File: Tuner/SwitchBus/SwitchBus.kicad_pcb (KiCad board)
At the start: 2 copper layers, 100 x 100 mm, 80 parts, among them J1 Conn_01x01, J10 Conn_Coaxial, J11 Conn_Coaxial, J12 Conn_Coaxial, J13 Conn_01x01, J14 Conn_01x01, J15 Conn_01x01, J16 Conn_Coaxial, J17 Conn_02x10_Odd_Even, J2 Conn_Coaxial, J3 Conn_Coaxial, J4 Conn_Coaxial, J5 Conn_Coaxial, J6 Conn_Coaxial, J7 Conn_Coaxial, J8 Conn_Coaxial, J9 Conn_Coaxial

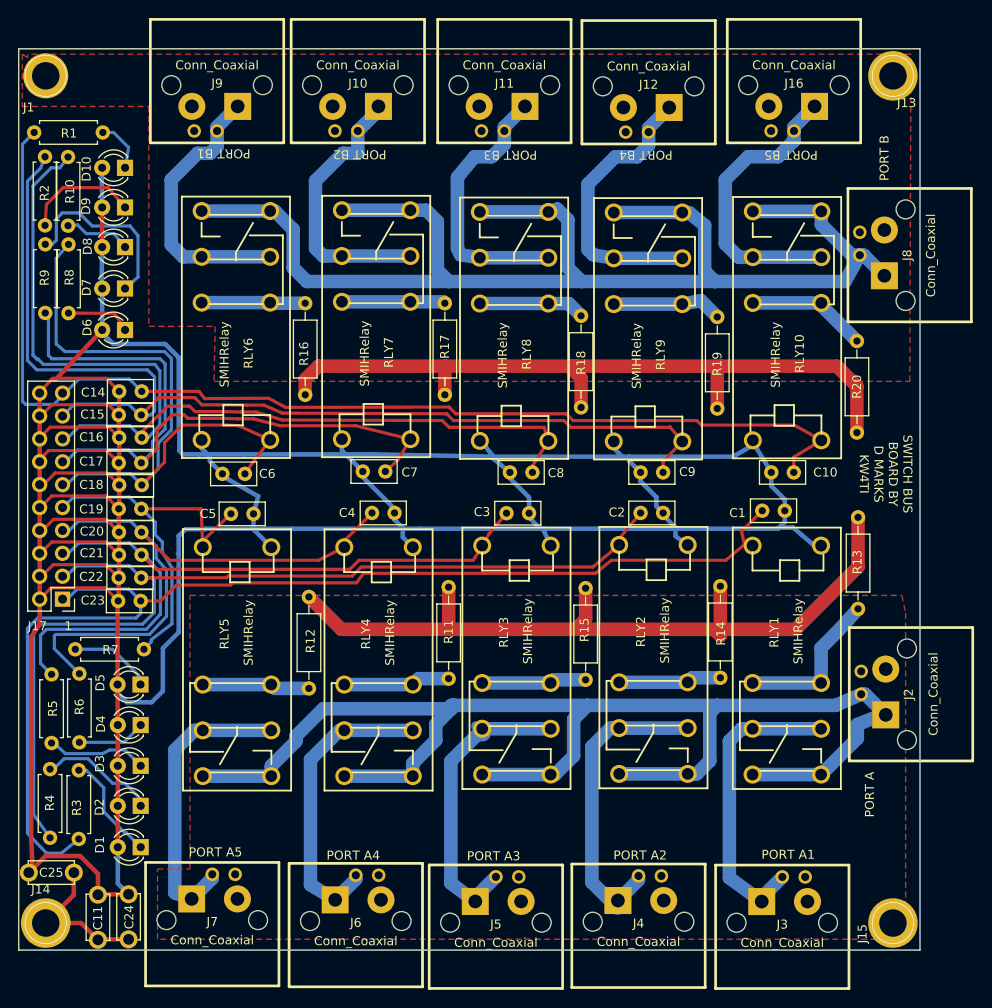
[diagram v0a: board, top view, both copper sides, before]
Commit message: Documentation update
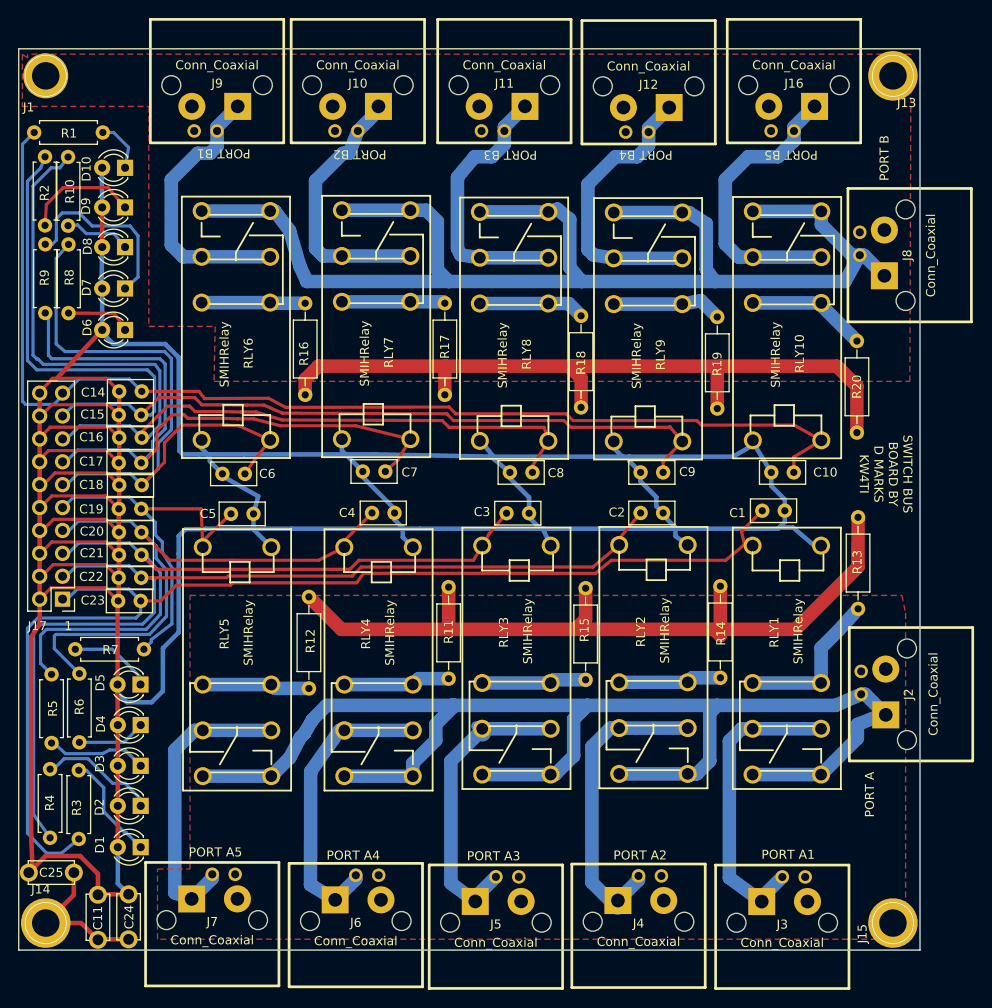
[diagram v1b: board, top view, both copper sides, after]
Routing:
- net Net-(J10-Pad1): track 30.5 -> 29.7 mm
- net Net-(J8-Pad1): track 152.8 -> 152.3 mm
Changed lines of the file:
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@@
   (segment (start 53 147) (end 56.9316 147) (width 0.5) (layer F.Cu) (net 22) (status 10))
   (segment (start 56.9316 147) (end 58.79084 148.85924) (width 0.5) (layer F.Cu) (net 22) (status 20))
-  (segment (start 78.025 130.7) (end 78.025 129.575) (width 1.5) (layer B.Cu) (net 23))
-  (segment (start 98.005 123.22) (end 98.005 122.85) (width 1.5) (layer B.Cu) (net 23))
-  (segment (start 83.81 123.22) (end 98.005 123.22) (width 1.5) (layer B.Cu) (net 23))
-  (segment (start 80.75 126.28) (end 83.81 123.22) (width 1.5) (layer B.Cu) (net 23))
-  (segment (start 80.75 126.85) (end 80.75 126.28) (width 1.5) (layer B.Cu) (net 23))
-  (segment (start 78.025 129.575) (end 80.75 126.85) (width 1.5) (layer B.Cu) (net 23))
+  (segment (start 98.375 122.85) (end 84.1473 122.85) (width 1.5) (layer B.Cu) (net 23))
+  (segment (start 80.0862 128.6388) (end 78.025 130.7) (width 1.5) (layer B.Cu) (net 23))
+  (segment (start 81.2546 126.4031) (end 80.0862 128.6388) (width 1.5) (layer B.Cu) (net 23))
+  (segment (start 81.7118 125.9459) (end 81.2546 126.4031) (width 1.5) (layer B.Cu) (net 23))
+  (segment (start 82.6008 124.4346) (end 81.7118 125.9459) (width 1.5) (layer B.Cu) (net 23))
+  (segment (start 84.1473 122.85) (end 82.6008 124.4346) (width 1.5) (layer B.Cu) (net 23))
   (segment (start 93.725 130.7) (end 93.725 129.275) (width 1.5) (layer B.Cu) (net 23))
   (segment (start 93.725 129.275) (end 96.275 126.725) (width 1.5) (layer B.Cu) (net 23))
@@
   (segment (start 87.4014 142.1384) (end 85.1154 144.4244) (width 1.5) (layer B.Cu) (net 28) (status 30))
   (segment (start 86.125 125.62) (end 85.605 125.62) (width 1.5) (layer B.Cu) (net 28))
-  (segment (start 85.605 125.62) (end 82.375 128.85) (width 1.5) (layer B.Cu) (net 28))
+  (segment (start 85.605 125.62) (end 82.3976 130.1877) (width 1.5) (layer B.Cu) (net 28))
   (segment (start 82.375 142.759) (end 85.1154 144.4244) (width 1.5) (layer B.Cu) (net 28) (status 20))
-  (segment (start 82.375 128.85) (end 82.375 142.759) (width 1.5) (layer B.Cu) (net 28))
+  (segment (start 82.3976 130.1877) (end 82.375 142.759) (width 1.5) (layer B.Cu) (net 28))
   (segment (start 86.125 125.62) (end 86.125 125.7) (width 2) (layer B.Cu) (net 28) (status 30))
   (segment (start 86.314 125.273) (end 86.68216 125.273) (width 1) (layer B.Cu) (net 28) (status 30))
@@
   (segment (start 142.4305 72.898) (end 139.055 69.5225) (width 1.5) (layer B.Cu) (net 30))
   (segment (start 77.9 68) (end 78.414 68) (width 1.5) (layer B.Cu) (net 30))
-  (segment (start 78.414 68) (end 80.4545 70.0405) (width 1.5) (layer B.Cu) (net 30))
+  (segment (start 78.414 68) (end 80.0481 70.1548) (width 1.5) (layer B.Cu) (net 30))
   (segment (start 81.9785 75.819) (end 97.7265 75.819) (width 1.5) (layer B.Cu) (net 30))
-  (segment (start 80.4545 74.295) (end 81.9785 75.819) (width 1.5) (layer B.Cu) (net 30))
-  (segment (start 80.4545 70.0405) (end 80.4545 74.295) (width 1.5) (layer B.Cu) (net 30))
+  (segment (start 81.2165 74.1553) (end 81.9785 75.819) (width 1.5) (layer B.Cu) (net 30))
+  (segment (start 80.0481 70.1548) (end 81.2165 74.1553) (width 1.5) (layer B.Cu) (net 30))
   (segment (start 93.462 67.912) (end 95.217 67.912) (width 1.5) (layer B.Cu) (net 30))
   (segment (start 97.7265 75.819) (end 112.4585 75.819) (width 1.5) (layer B.Cu) (net 30))
@@
   (segment (start 95.217 67.912) (end 96.4565 69.1515) (width 1.5) (layer B.Cu) (net 30))
   (segment (start 108.7655 68.1025) (end 109.7585 67.785) (width 1.5) (layer B.Cu) (net 30) (status 10))
-  (segment (start 109.7585 67.785) (end 110.9345 68.961) (width 1.5) (layer B.Cu) (net 30))
-  (segment (start 110.9345 68.961) (end 110.9345 74.295) (width 1.5) (layer B.Cu) (net 30))
-  (segment (start 110.9345 74.295) (end 112.4585 75.819) (width 1.5) (layer B.Cu) (net 30))
+  (segment (start 109.7585 67.785) (end 111.1377 68.9229) (width 1.5) (layer B.Cu) (net 30))
+  (segment (start 111.1377 68.9229) (end 111.1377 74.2569) (width 1.5) (layer B.Cu) (net 30))
+  (segment (start 111.1377 74.2569) (end 112.4585 75.819) (width 1.5) (layer B.Cu) (net 30))
   (segment (start 112.4585 75.819) (end 127.254 75.819) (width 1.5) (layer B.Cu) (net 30))
   (segment (start 123.6245 68.166) (end 124.3635 68.166) (width 1.5) (layer B.Cu) (net 30) (status 30))
-  (segment (start 124.3635 68.166) (end 126.111 69.596) (width 1.5) (layer B.Cu) (net 30) (status 10))
-  (segment (start 126.111 69.596) (end 126.111 74.676) (width 1.5) (layer B.Cu) (net 30))
-  (segment (start 126.111 74.676) (end 127.254 75.819) (width 1.5) (layer B.Cu) (net 30))
+  (segment (start 124.3635 68.166) (end 126.2888 69.4055) (width 1.5) (layer B.Cu) (net 30) (status 10))
+  (segment (start 126.2888 69.4055) (end 126.2888 74.4855) (width 1.5) (layer B.Cu) (net 30))
+  (segment (start 126.2888 74.4855) (end 127.254 75.819) (width 1.5) (layer B.Cu) (net 30))
   (segment (start 141.671 75.819) (end 143.322 72.898) (width 1.5) (layer B.Cu) (net 30) (status 20))
   (segment (start 127.254 75.819) (end 141.671 75.819) (width 1.5) (layer B.Cu) (net 30))
@@
   (segment (start 89.916 56.83) (end 87.63 59.116) (width 1.5) (layer B.Cu) (net 37))
   (segment (start 85.862 72.992) (end 83.787 72.992) (width 1.5) (layer B.Cu) (net 37))
-  (segment (start 87.63 61.595) (end 87.63 59.116) (width 1.5) (layer B.Cu) (net 37))
-  (segment (start 85.979 61.595) (end 87.63 61.595) (width 1.5) (layer B.Cu) (net 37))
+  (segment (start 86.6648 61.58992) (end 87.63 59.116) (width 1.5) (layer B.Cu) (net 37) (status 800000))
+  (segment (start 85.979 61.595) (end 86.6648 61.58992) (width 1.5) (layer B.Cu) (net 37))
   (segment (start 82.931 64.643) (end 85.979 61.595) (width 1.5) (layer B.Cu) (net 37))
   (segment (start 82.931 72.136) (end 82.931 64.643) (width 1.5) (layer B.Cu) (net 37))

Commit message: Added some fixes to tuner code
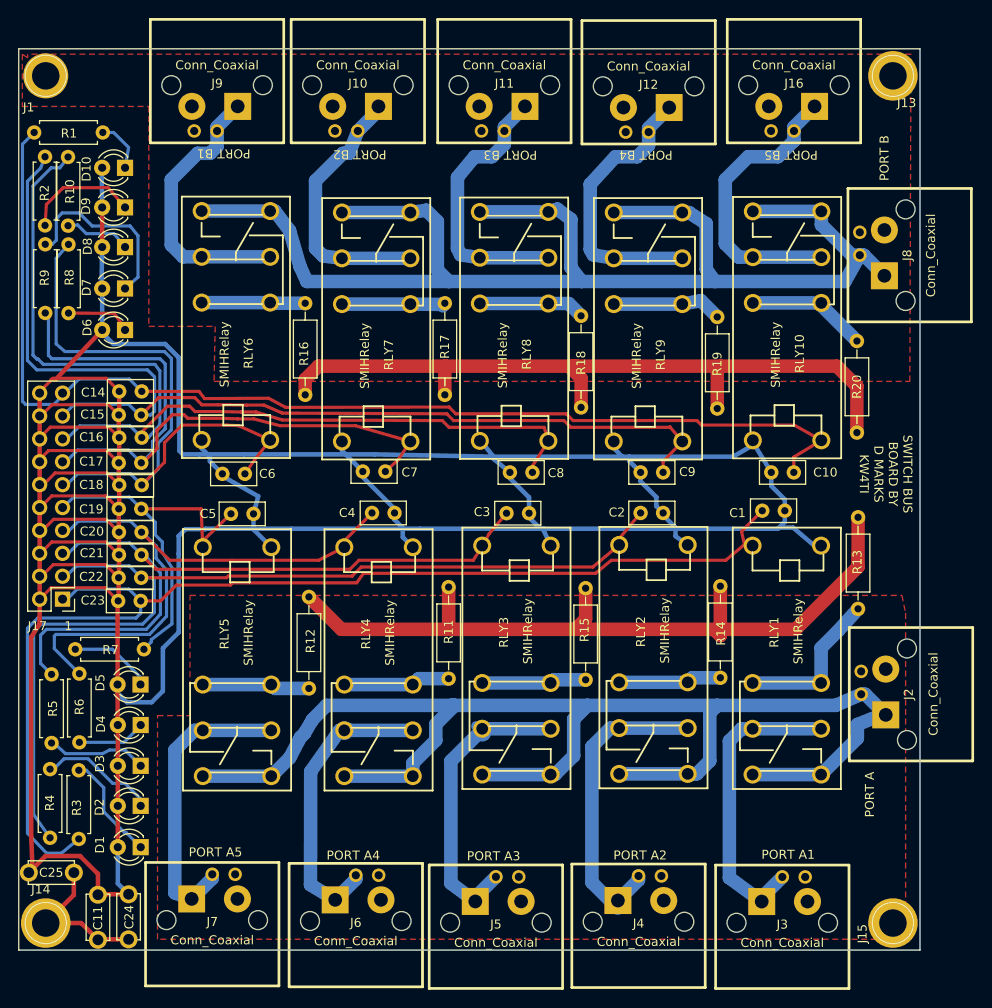
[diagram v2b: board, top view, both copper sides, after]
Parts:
- moved RLY7 0.25 mm to (89.7, 83.6)
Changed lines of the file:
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@@
   )
   (setup
-    (last_trace_width 1.5)
+    (last_trace_width 0.25)
     (user_trace_width 0.35)
     (user_trace_width 0.5)
@@
   )
   (module tuner:SMIHRelay (layer F.Cu)
-    (at 89.662 83.312 90)
+    (at 89.662 83.566 90)
     (fp_text reference RLY7 (at -0.381 1.397 90) (layer F.SilkS)
       (effects (font (size 1 1) (thickness 0.15)))
@@
   (segment (start 76.073 91.059) (end 78.994 91.821) (width 0.35) (layer F.Cu) (net 7))
   (segment (start 90.678 96.901) (end 92.075 95.631) (width 0.35) (layer F.Cu) (net 7) (status 10))
-  (segment (start 92.075 95.631) (end 93.462 93.312) (width 0.35) (layer F.Cu) (net 7) (status 20))
-  (segment (start 87.376 91.821) (end 93.462 93.312) (width 0.35) (layer F.Cu) (net 7) (status 20))
+  (segment (start 92.075 95.631) (end 93.462 93.566) (width 0.35) (layer F.Cu) (net 7) (status 20))
+  (segment (start 87.376 91.821) (end 93.462 93.566) (width 0.35) (layer F.Cu) (net 7) (status 20))
   (segment (start 72.62 91) (end 74.295 91.059) (width 0.35) (layer F.Cu) (net 7))
   (segment (start 52.9463 79.3115) (end 52.9463 79.2861) (width 0.35) (layer F.Cu) (net 7) (status 30))
@@
   (segment (start 104.5 97.642) (end 104.5 97) (width 0.5) (layer B.Cu) (net 9))
   (segment (start 106.625 101.525) (end 106.625 101.625) (width 0.5) (layer B.Cu) (net 9))
-  (segment (start 85.862 93.312) (end 85.862 94.585) (width 0.5) (layer B.Cu) (net 9))
+  (segment (start 85.862 93.566) (end 85.862 94.585) (width 0.5) (layer B.Cu) (net 9) (status 10))
   (segment (start 85.862 94.585) (end 88.178 96.901) (width 0.5) (layer B.Cu) (net 9))
   (segment (start 71.21 95.25) (end 71.21 95.77) (width 0.5) (layer B.Cu) (net 9))
@@
   (segment (start 81.2165 74.1553) (end 81.9785 75.819) (width 1.5) (layer B.Cu) (net 30))
   (segment (start 80.0481 70.1548) (end 81.2165 74.1553) (width 1.5) (layer B.Cu) (net 30))
-  (segment (start 93.462 67.912) (end 95.217 67.912) (width 1.5) (layer B.Cu) (net 30))
+  (segment (start 93.462 68.166) (end 95.217 67.912) (width 1.5) (layer B.Cu) (net 30) (status 10))
   (segment (start 97.7265 75.819) (end 112.4585 75.819) (width 1.5) (layer B.Cu) (net 30))
   (segment (start 96.4565 74.549) (end 97.7265 75.819) (width 1.5) (layer B.Cu) (net 30))
@@
   (segment (start 95.217 67.912) (end 96.4565 69.1515) (width 1.5) (layer B.Cu) (net 30))
   (segment (start 108.7655 68.1025) (end 109.7585 67.785) (width 1.5) (layer B.Cu) (net 30) (status 10))
-  (segment (start 109.7585 67.785) (end 111.1377 68.9229) (width 1.5) (layer B.Cu) (net 30))
-  (segment (start 111.1377 68.9229) (end 111.1377 74.2569) (width 1.5) (layer B.Cu) (net 30))
-  (segment (start 111.1377 74.2569) (end 112.4585 75.819) (width 1.5) (layer B.Cu) (net 30))
+  (segment (start 109.7585 67.785) (end 111.2647 68.9229) (width 1.5) (layer B.Cu) (net 30))
+  (segment (start 111.2647 68.9229) (end 111.2647 74.2569) (width 1.5) (layer B.Cu) (net 30))
+  (segment (start 111.2647 74.2569) (end 112.4585 75.819) (width 1.5) (layer B.Cu) (net 30))
   (segment (start 112.4585 75.819) (end 127.254 75.819) (width 1.5) (layer B.Cu) (net 30))
   (segment (start 123.6245 68.166) (end 124.3635 68.166) (width 1.5) (layer B.Cu) (net 30) (status 30))
@@
   (segment (start 116.0245 68.166) (end 123.6245 68.166) (width 1.5) (layer B.Cu) (net 30) (status 30))
   (segment (start 101.1655 68.1025) (end 108.7655 68.1025) (width 1.5) (layer B.Cu) (net 30) (status 30))
-  (segment (start 85.862 67.912) (end 93.462 67.912) (width 1.5) (layer B.Cu) (net 30))
+  (segment (start 85.862 68.166) (end 93.462 68.166) (width 1.5) (layer B.Cu) (net 30) (status 30))
   (segment (start 70.3 68) (end 77.9 68) (width 1.5) (layer B.Cu) (net 30))
   (segment (start 97.7 119.885) (end 94.38 119.885) (width 1.5) (layer B.Cu) (net 31))
@@
   (segment (start 66.929 71.755) (end 66.929 64.516) (width 1.5) (layer B.Cu) (net 36))
   (segment (start 68.254 73.08) (end 66.929 71.755) (width 1.5) (layer B.Cu) (net 36))
-  (segment (start 93.462 72.992) (end 85.862 72.992) (width 1.5) (layer B.Cu) (net 37))
+  (segment (start 93.462 73.246) (end 85.862 73.246) (width 1.5) (layer B.Cu) (net 37) (status 30))
   (segment (start 89.916 56.388) (end 89.916 56.83) (width 1.5) (layer B.Cu) (net 37))
   (segment (start 89.916 56.83) (end 87.63 59.116) (width 1.5) (layer B.Cu) (net 37))
-  (segment (start 85.862 72.992) (end 83.787 72.992) (width 1.5) (layer B.Cu) (net 37))
-  (segment (start 86.6648 61.58992) (end 87.63 59.116) (width 1.5) (layer B.Cu) (net 37) (status 800000))
+  (segment (start 85.862 73.246) (end 83.787 72.992) (width 1.5) (layer B.Cu) (net 37) (status 10))
+  (segment (start 86.6648 61.58992) (end 87.63 59.116) (width 1.5) (layer B.Cu) (net 37))
   (segment (start 85.979 61.595) (end 86.6648 61.58992) (width 1.5) (layer B.Cu) (net 37))
   (segment (start 82.931 64.643) (end 85.979 61.595) (width 1.5) (layer B.Cu) (net 37))
@@
   (segment (start 118.618 61.976) (end 119.888 60.706) (width 1.5) (layer B.Cu) (net 39))
   (segment (start 116.205 61.976) (end 118.618 61.976) (width 1.5) (layer B.Cu) (net 39))
-  (segment (start 113.157 65.024) (end 116.205 61.976) (width 1.5) (layer B.Cu) (net 39))
-  (segment (start 113.157 72.263) (end 113.157 65.024) (width 1.5) (layer B.Cu) (net 39))
-  (segment (start 113.759 72.865) (end 113.157 72.263) (width 1.5) (layer B.Cu) (net 39))
+  (segment (start 113.411 65.024) (end 116.205 61.976) (width 1.5) (layer B.Cu) (net 39))
+  (segment (start 113.411 72.263) (end 113.411 65.024) (width 1.5) (layer B.Cu) (net 39))
+  (segment (start 113.759 72.865) (end 113.411 72.263) (width 1.5) (layer B.Cu) (net 39))
   (segment (start 139.055 73.119) (end 131.455 73.119) (width 1.5) (layer B.Cu) (net 40))
   (segment (start 136.017 59.116) (end 136.017 58.674) (width 1.5) (layer B.Cu) (net 40))
@@
   (segment (start 77.972 78.232) (end 77.9 78.16) (width 1.5) (layer B.Cu) (net 41))
   (segment (start 70.3 78.16) (end 77.9 78.16) (width 1.5) (layer B.Cu) (net 41))
-  (segment (start 93.462 78.072) (end 97.122 78.072) (width 1.5) (layer B.Cu) (net 42))
-  (segment (start 97.122 78.072) (end 97.282 78.232) (width 1.5) (layer B.Cu) (net 42))
-  (segment (start 85.862 78.072) (end 93.462 78.072) (width 1.5) (layer B.Cu) (net 42))
+  (segment (start 93.462 78.326) (end 96.901 78.359) (width 1.5) (layer B.Cu) (net 42) (status 10))
+  (segment (start 96.901 78.359) (end 97.061 78.519) (width 1.5) (layer B.Cu) (net 42))
+  (segment (start 85.862 78.326) (end 93.462 78.326) (width 1.5) (layer B.Cu) (net 42) (status 30))
   (segment (start 108.7655 78.2625) (end 111.0285 78.2625) (width 1.5) (layer B.Cu) (net 43))
   (segment (start 111.0285 78.2625) (end 112.395 79.629) (width 1.5) (layer B.Cu) (net 43))
@@
     (polygon
       (pts
-        (xy 148.4 112.6) (xy 148.4 148.8) (xy 65.4 148.8) (xy 65.4 141) (xy 69 141)
+        (xy 148.4 112.6) (xy 148.4 148.8) (xy 65.4 148.8) (xy 65.4 123.982) (xy 69 123.982)
         (xy 69 110.65) (xy 148 110.65)
       )
